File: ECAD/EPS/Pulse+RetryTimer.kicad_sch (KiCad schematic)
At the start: 13 parts, among them Q16 2N7002, Q17 2N7002, U16 LM321, U17 LTC6993xS6-4

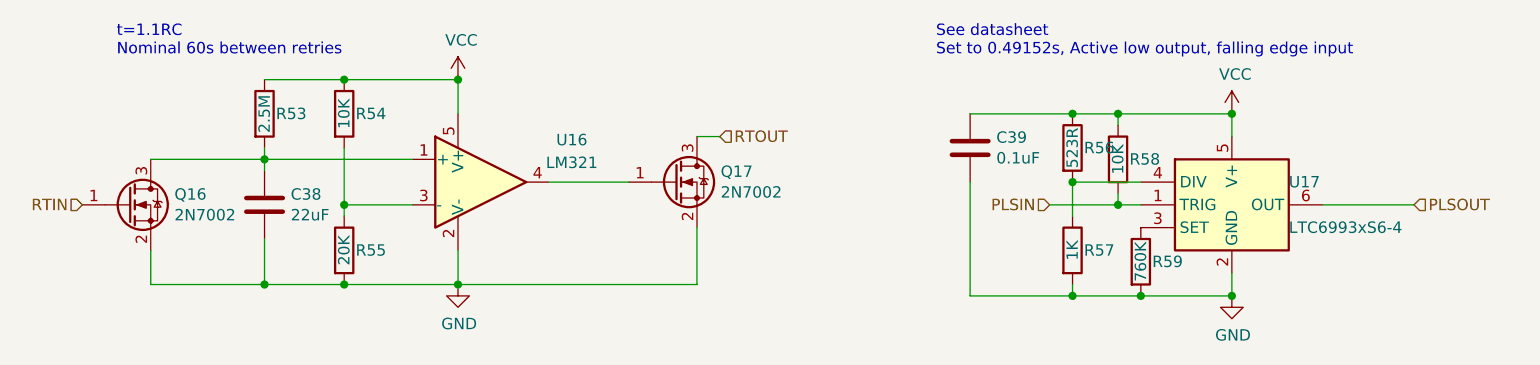
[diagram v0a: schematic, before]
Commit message: Revert "Micro + PCM blocks"
This reverts commit bd53ca95fb26b4e6798500a23db46c8297649bcb.
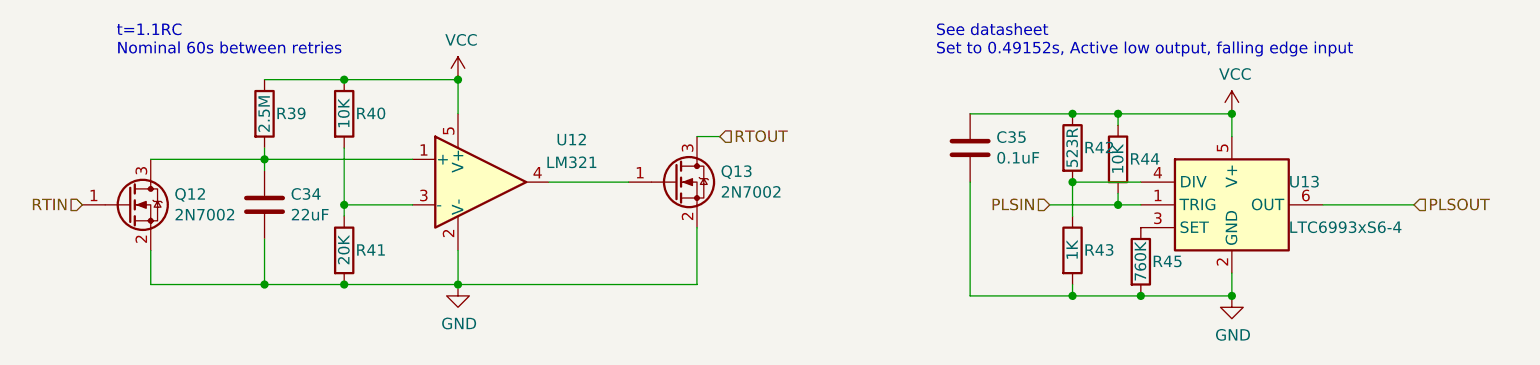
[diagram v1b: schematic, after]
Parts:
- renumbered C38 to C34, C39 to C35, Q16 to Q12, Q17 to Q13, R53 to R39, R54 to R40, R55 to R41, R56 to R42, R57 to R43, R58 to R44, R59 to R45, U16 to U12, U17 to U13
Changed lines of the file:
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@@
     (effects (font (size 1.27 1.27)) (justify right))
   )
-  (symbol (lib_id "Transistor_FET:2N7002") (at 38.1 43.18 0)
-    (in_bom yes) (on_board yes)
-    (property "Reference" "Q16" (id 0) (at 43.2816 42.0116 0)
+  (symbol (lib_id "Transistor_FET:2N7002") (at 38.1 43.18 0) (unit 1)
+    (in_bom yes) (on_board yes)
+    (property "Reference" "Q12" (id 0) (at 43.2816 42.0116 0)
       (effects (font (size 1.27 1.27)) (justify left))
     )
@@
     (pin "3")
   )
-  (symbol (lib_id "Transistor_FET:2N7002") (at 99.06 40.64 0)
-    (in_bom yes) (on_board yes)
-    (property "Reference" "Q17" (id 0) (at 104.2416 39.4716 0)
+  (symbol (lib_id "Transistor_FET:2N7002") (at 99.06 40.64 0) (unit 1)
+    (in_bom yes) (on_board yes)
+    (property "Reference" "Q13" (id 0) (at 104.2416 39.4716 0)
       (effects (font (size 1.27 1.27)) (justify left))
     )
@@
     (pin "3")
   )
-  (symbol (lib_id "Device:R") (at 62.23 33.02 0)
-    (in_bom yes) (on_board yes)
-    (property "Reference" "R54" (id 0) (at 63.5 33.02 0)
+  (symbol (lib_id "Device:R") (at 62.23 33.02 0) (unit 1)
+    (in_bom yes) (on_board yes)
+    (property "Reference" "R40" (id 0) (at 63.5 33.02 0)
       (effects (font (size 1.27 1.27)) (justify left))
     )
@@
     (pin "2")
   )
-  (symbol (lib_id "Device:R") (at 62.23 48.26 0)
-    (in_bom yes) (on_board yes)
-    (property "Reference" "R55" (id 0) (at 63.5 48.26 0)
+  (symbol (lib_id "Device:R") (at 62.23 48.26 0) (unit 1)
+    (in_bom yes) (on_board yes)
+    (property "Reference" "R41" (id 0) (at 63.5 48.26 0)
       (effects (font (size 1.27 1.27)) (justify left))
     )
@@
     (pin "2")
   )
-  (symbol (lib_id "power:VCC") (at 74.93 29.21 0)
-    (in_bom yes) (on_board yes)
-    (property "Reference" "#PWR064" (id 0) (at 74.93 33.02 0)
+  (symbol (lib_id "power:VCC") (at 74.93 29.21 0) (unit 1)
+    (in_bom yes) (on_board yes)
+    (property "Reference" "#PWR056" (id 0) (at 74.93 33.02 0)
       (effects (font (size 1.27 1.27)) hide)
     )
@@
     (pin "1")
   )
-  (symbol (lib_id "Device:R") (at 53.34 33.02 0)
-    (in_bom yes) (on_board yes)
-    (property "Reference" "R53" (id 0) (at 54.61 33.02 0)
+  (symbol (lib_id "Device:R") (at 53.34 33.02 0) (unit 1)
+    (in_bom yes) (on_board yes)
+    (property "Reference" "R39" (id 0) (at 54.61 33.02 0)
       (effects (font (size 1.27 1.27)) (justify left))
     )
@@
     (pin "2")
   )
-  (symbol (lib_id "Device:C") (at 53.34 43.18 0)
-    (in_bom yes) (on_board yes)
-    (property "Reference" "C38" (id 0) (at 56.261 42.0116 0)
+  (symbol (lib_id "Device:C") (at 53.34 43.18 0) (unit 1)
+    (in_bom yes) (on_board yes)
+    (property "Reference" "C34" (id 0) (at 56.261 42.0116 0)
       (effects (font (size 1.27 1.27)) (justify left))
     )
@@
     (pin "2")
   )
-  (symbol (lib_id "power:GND") (at 74.93 52.07 0)
-    (in_bom yes) (on_board yes)
-    (property "Reference" "#PWR065" (id 0) (at 74.93 58.42 0)
+  (symbol (lib_id "power:GND") (at 74.93 52.07 0) (unit 1)
+    (in_bom yes) (on_board yes)
+    (property "Reference" "#PWR057" (id 0) (at 74.93 58.42 0)
       (effects (font (size 1.27 1.27)) hide)
     )
@@
     (pin "1")
   )
-  (symbol (lib_id "Timer:LTC6993xS6-4") (at 161.29 43.18 0)
-    (in_bom yes) (on_board yes)
-    (property "Reference" "U17" (id 0) (at 167.64 40.64 0)
+  (symbol (lib_id "Timer:LTC6993xS6-4") (at 161.29 43.18 0) (unit 1)
+    (in_bom yes) (on_board yes)
+    (property "Reference" "U13" (id 0) (at 167.64 40.64 0)
       (effects (font (size 1.27 1.27)) (justify left))
     )
@@
     (pin "6")
   )
-  (symbol (lib_id "power:VCC") (at 161.29 33.02 0)
-    (in_bom yes) (on_board yes)
-    (property "Reference" "#PWR066" (id 0) (at 161.29 36.83 0)
+  (symbol (lib_id "power:VCC") (at 161.29 33.02 0) (unit 1)
+    (in_bom yes) (on_board yes)
+    (property "Reference" "#PWR058" (id 0) (at 161.29 36.83 0)
       (effects (font (size 1.27 1.27)) hide)
     )
@@
     (pin "1")
   )
-  (symbol (lib_id "Device:R") (at 143.51 48.26 0)
-    (in_bom yes) (on_board yes)
-    (property "Reference" "R57" (id 0) (at 144.78 48.26 0)
+  (symbol (lib_id "Device:R") (at 143.51 48.26 0) (unit 1)
+    (in_bom yes) (on_board yes)
+    (property "Reference" "R43" (id 0) (at 144.78 48.26 0)
       (effects (font (size 1.27 1.27)) (justify left))
     )
@@
     (pin "2")
   )
-  (symbol (lib_id "Device:R") (at 143.51 36.83 0)
-    (in_bom yes) (on_board yes)
-    (property "Reference" "R56" (id 0) (at 144.78 36.83 0)
+  (symbol (lib_id "Device:R") (at 143.51 36.83 0) (unit 1)
+    (in_bom yes) (on_board yes)
+    (property "Reference" "R42" (id 0) (at 144.78 36.83 0)
       (effects (font (size 1.27 1.27)) (justify left))
     )
@@
     (pin "2")
   )
-  (symbol (lib_id "Device:R") (at 151.13 49.53 0)
-    (in_bom yes) (on_board yes)
-    (property "Reference" "R59" (id 0) (at 152.4 49.53 0)
+  (symbol (lib_id "Device:R") (at 151.13 49.53 0) (unit 1)
+    (in_bom yes) (on_board yes)
+    (property "Reference" "R45" (id 0) (at 152.4 49.53 0)
       (effects (font (size 1.27 1.27)) (justify left))
     )
@@
     (pin "2")
   )
-  (symbol (lib_id "Device:C") (at 132.08 36.83 0)
-    (in_bom yes) (on_board yes)
-    (property "Reference" "C39" (id 0) (at 135.001 35.6616 0)
+  (symbol (lib_id "Device:C") (at 132.08 36.83 0) (unit 1)
+    (in_bom yes) (on_board yes)
+    (property "Reference" "C35" (id 0) (at 135.001 35.6616 0)
       (effects (font (size 1.27 1.27)) (justify left))
     )
@@
     (pin "2")
   )
-  (symbol (lib_id "Device:R") (at 148.59 38.1 0)
-    (in_bom yes) (on_board yes)
-    (property "Reference" "R58" (id 0) (at 149.86 38.1 0)
+  (symbol (lib_id "Device:R") (at 148.59 38.1 0) (unit 1)
+    (in_bom yes) (on_board yes)
+    (property "Reference" "R44" (id 0) (at 149.86 38.1 0)
       (effects (font (size 1.27 1.27)) (justify left))
     )
@@
     (pin "2")
   )
-  (symbol (lib_id "power:GND") (at 161.29 53.34 0)
-    (in_bom yes) (on_board yes)
-    (property "Reference" "#PWR067" (id 0) (at 161.29 59.69 0)
+  (symbol (lib_id "power:GND") (at 161.29 53.34 0) (unit 1)
+    (in_bom yes) (on_board yes)
+    (property "Reference" "#PWR059" (id 0) (at 161.29 59.69 0)
       (effects (font (size 1.27 1.27)) hide)
     )
@@
     (pin "1")
   )
-  (symbol (lib_id "Amplifier_Operational:LM321") (at 77.47 40.64 0)
+  (symbol (lib_id "Amplifier_Operational:LM321") (at 77.47 40.64 0) (unit 1)
     (in_bom yes) (on_board yes) (fields_autoplaced)
-    (property "Reference" "U16" (id 0) (at 87.63 35.941 0))
+    (property "Reference" "U12" (id 0) (at 87.63 35.941 0))
     (property "Value" "LM321" (id 1) (at 87.63 38.481 0))
     (property "Footprint" "Package_TO_SOT_SMD:SOT-23-5" (id 2) (at 77.47 40.64 0)
